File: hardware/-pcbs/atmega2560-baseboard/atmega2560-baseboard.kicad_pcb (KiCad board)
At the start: 2 copper layers, 18 parts, among them J1 Bottom, SW1 SW_Push, U1 ATMEGA2560-16AU, Y1 16MHz

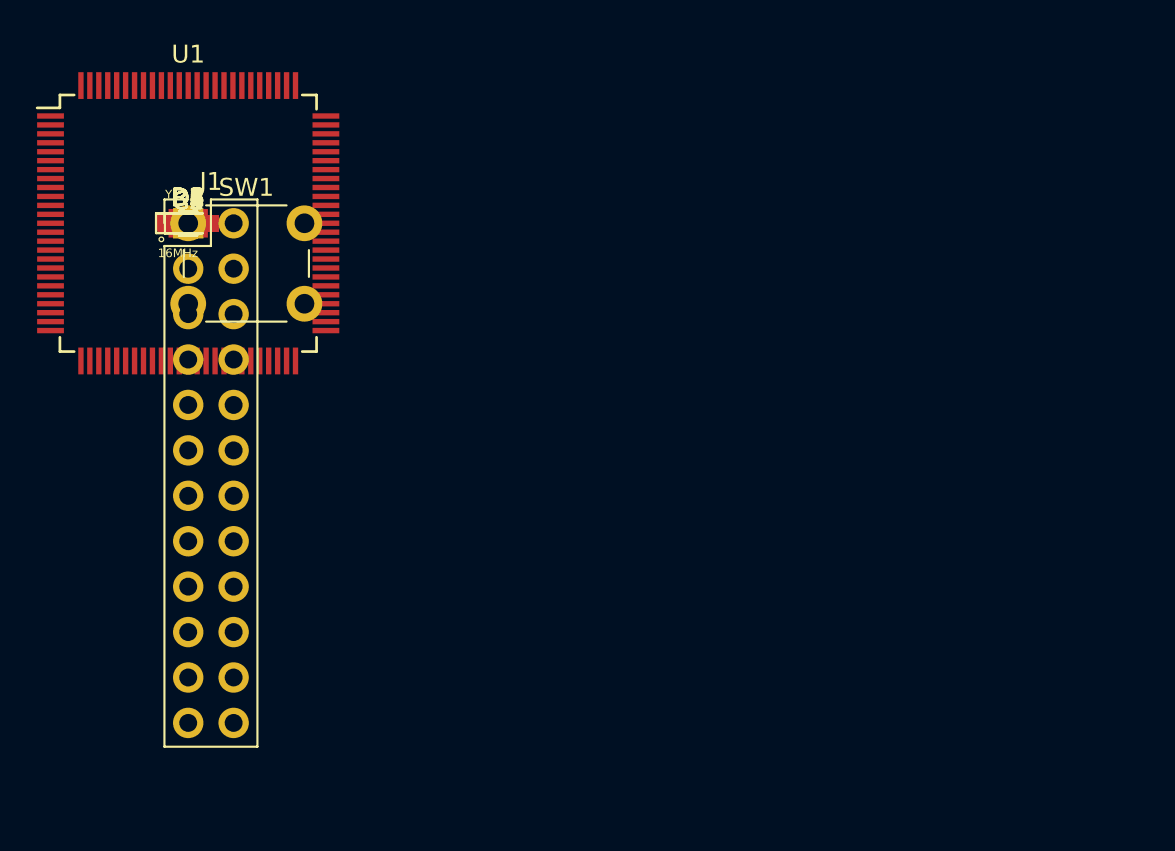
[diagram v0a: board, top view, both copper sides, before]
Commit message: Spread out all footprints
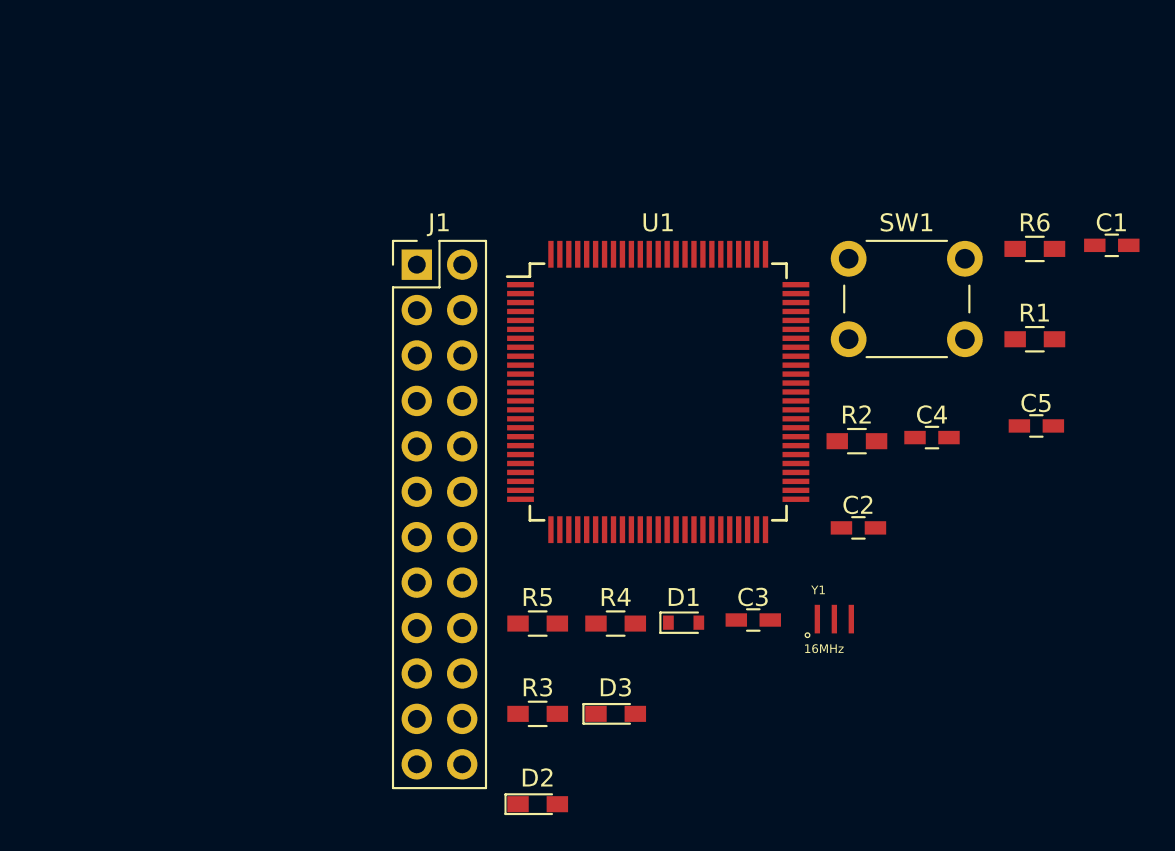
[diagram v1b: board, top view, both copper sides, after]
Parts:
- moved C1 51.7 mm to (200.1, 106.2)
- moved C5 48.8 mm to (195.9, 116.3)
- moved R1 47.8 mm to (195.8, 111.5)
- moved R6 47.4 mm to (195.8, 106.4)
- moved C4 43.3 mm to (190.1, 117.0)
- moved Y1 42.4 mm to (184.6, 127.1)
- moved C2 41.2 mm to (186.0, 122.0)
- moved R2 39.3 mm to (185.9, 117.2)
- moved C3 38.6 mm to (180.1, 127.2)
- moved D2 37.9 mm to (168.0, 137.5)
- moved SW1 37.0 mm to (185.4, 107.0)
- moved D3 36.4 mm to (172.4, 132.4)
- moved D1 35.6 mm to (176.2, 127.3)
- moved R3 33.7 mm to (168.0, 132.4)
- moved R4 32.7 mm to (172.4, 127.4)
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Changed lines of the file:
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@@
   (general
     (links 62)
-    (no_connects 47)
+    (no_connects 62)
     (area 0 0 0 0)
     (thickness 1.6)
@@
   )
   (module Capacitors_SMD:C_0603_HandSoldering (layer F.Cu)
-    (at 148.5011 105.0036)
+    (at 200.146571 106.238)
     (descr "Capacitor SMD 0603, hand soldering")
     (tags "capacitor 0603")
@@
   )
   (module Capacitors_SMD:C_0603_HandSoldering (layer F.Cu)
-    (at 148.5011 105.0036)
+    (at 185.979428 122.038)
     (descr "Capacitor SMD 0603, hand soldering")
     (tags "capacitor 0603")
@@
   )
   (module Capacitors_SMD:C_0603_HandSoldering (layer F.Cu)
-    (at 148.5011 105.0036)
+    (at 180.099428 127.188)
     (descr "Capacitor SMD 0603, hand soldering")
     (tags "capacitor 0603")
@@
   )
   (module Capacitors_SMD:C_0603_HandSoldering (layer F.Cu)
-    (at 148.5011 105.0036)
+    (at 190.093001 116.988)
     (descr "Capacitor SMD 0603, hand soldering")
     (tags "capacitor 0603")
@@
   )
   (module Capacitors_SMD:C_0603_HandSoldering (layer F.Cu)
-    (at 148.5011 105.0036)
+    (at 195.929428 116.338)
     (descr "Capacitor SMD 0603, hand soldering")
     (tags "capacitor 0603")
@@
   )
   (module Diodes_SMD:D_0603 (layer F.Cu)
-    (at 148.5011 105.0036)
+    (at 176.203001 127.338)
     (descr "Diode SMD in 0603 package http://datasheets.avx.com/schottky.pdf")
     (tags "smd diode")
@@
   )
   (module LEDs:LED_0603_HandSoldering (layer F.Cu)
-    (at 148.5011 105.0036)
+    (at 168.043001 137.488)
     (descr "LED SMD 0603, hand soldering")
     (tags "LED 0603")
@@
   )
   (module LEDs:LED_0603_HandSoldering (layer F.Cu)
-    (at 148.5011 105.0036)
+    (at 172.403001 132.438)
     (descr "LED SMD 0603, hand soldering")
     (tags "LED 0603")
@@
   )
   (module Pin_Headers:Pin_Header_Straight_2x12_Pitch2.54mm (layer F.Cu)
-    (at 148.5011 105.0036)
+    (at 161.283001 107.318)
     (descr "Through hole straight pin header, 2x12, 2.54mm pitch, double rows")
     (tags "Through hole pin header THT 2x12 2.54mm double row")
@@
   )
   (module Resistors_SMD:R_0603_HandSoldering (layer F.Cu)
-    (at 148.5011 105.0036)
+    (at 195.843001 111.488)
     (descr "Resistor SMD 0603, hand soldering")
     (tags "resistor 0603")
@@
   )
   (module Resistors_SMD:R_0603_HandSoldering (layer F.Cu)
-    (at 148.5011 105.0036)
+    (at 185.893001 117.188)
     (descr "Resistor SMD 0603, hand soldering")
     (tags "resistor 0603")
@@
   )
   (module Resistors_SMD:R_0603_HandSoldering (layer F.Cu)
-    (at 148.5011 105.0036)
+    (at 168.043001 132.438)
     (descr "Resistor SMD 0603, hand soldering")
     (tags "resistor 0603")
@@
   )
   (module Resistors_SMD:R_0603_HandSoldering (layer F.Cu)
-    (at 148.5011 105.0036)
+    (at 172.403001 127.388)
     (descr "Resistor SMD 0603, hand soldering")
     (tags "resistor 0603")
@@
   )
   (module Resistors_SMD:R_0603_HandSoldering (layer F.Cu)
-    (at 148.5011 105.0036)
+    (at 168.043001 127.388)
     (descr "Resistor SMD 0603, hand soldering")
     (tags "resistor 0603")
@@
   )
   (module Resistors_SMD:R_0603_HandSoldering (layer F.Cu)
-    (at 148.5011 105.0036)
+    (at 195.843001 106.438)
     (descr "Resistor SMD 0603, hand soldering")
     (tags "resistor 0603")
@@
   )
   (module Buttons_Switches_THT:SW_PUSH_6mm (layer F.Cu)
-    (at 148.5011 105.0036)
+    (at 185.433001 106.988)
     (descr https://www.omron.com/ecb/products/pdf/en-b3f.pdf)
     (tags "tact sw push 6mm")
@@
   )
   (module Housings_QFP:TQFP-100_14x14mm_Pitch0.5mm (layer F.Cu)
-    (at 148.5011 105.0036)
+    (at 174.783001 114.438)
     (descr "100-Lead Plastic Thin Quad Flatpack (PF) - 14x14x1 mm Body 2.00 mm Footprint [TQFP] (see Microchip Packaging Specification 00000049BS.pdf)")
     (tags "QFP 0.5")
@@
   )
   (module CSTCE16M0V53-R0:OSC_CSTCE16M0V53-R0 (layer F.Cu)
-    (at 148.5011 105.0036)
+    (at 184.631501 127.138116)
     (attr smd)
     (fp_text reference Y1 (at -0.882758 -1.61337) (layer F.SilkS)
